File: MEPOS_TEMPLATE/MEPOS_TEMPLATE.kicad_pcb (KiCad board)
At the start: 4 copper layers, 101.6 x 101.6 mm, 10 parts, among them J201 Conn_02x32_Odd_Even, J202 Conn_02x20_Odd_Even

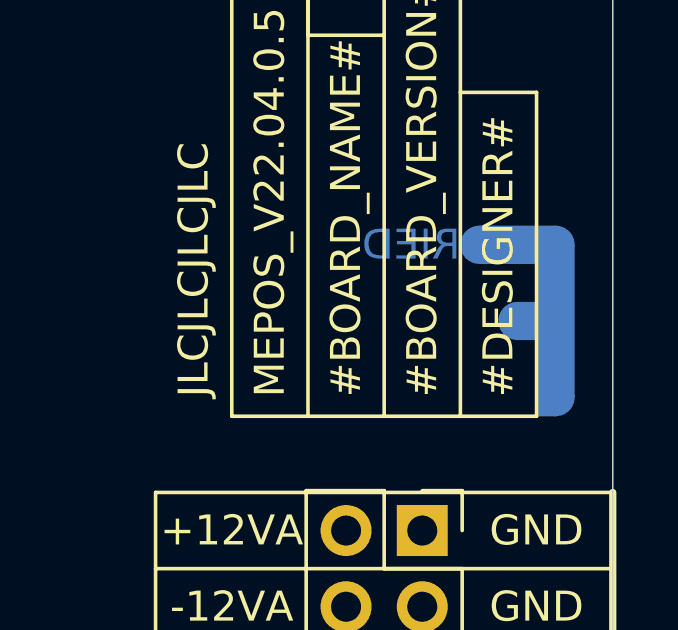
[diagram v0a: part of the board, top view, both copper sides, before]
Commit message: Updated Libraries
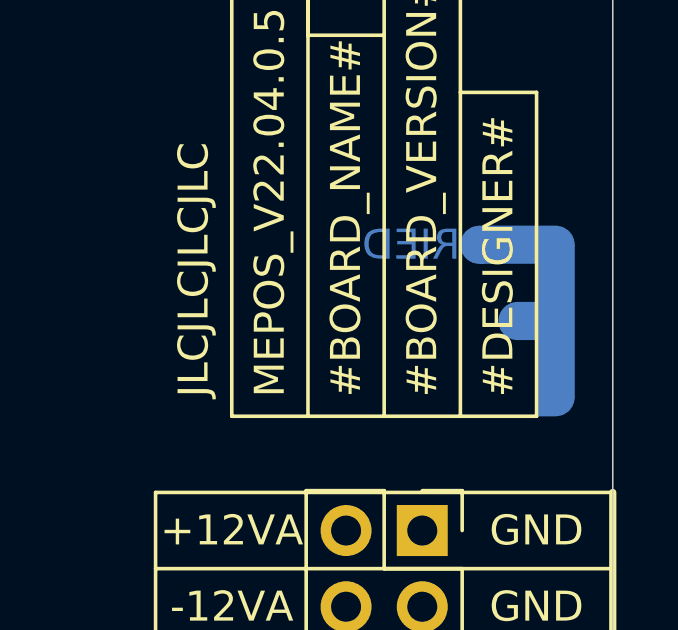
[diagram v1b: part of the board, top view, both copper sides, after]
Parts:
- removed the REF** at (188.1, 68.9)
- added REF**: Logo, MEPOS:Logo, F.Cu at (188.1, 68.9)
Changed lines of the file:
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@@
     )
   )
-  (footprint "MEP_TEMPLATE:Logo" (layer "F.Cu")
-    (at 188.09775 68.885)
+  (footprint "MEPOS:Logo" (layer "F.Cu")
+    (at 188.1 68.885)
     (attr smd)
     (fp_text reference "REF**" (at 0 -4.445 unlocked) (layer "F.Fab")
@@
     )
     (fp_circle (center 3.175 -2.54) (end 3.81 -2.54) (layer "B.Cu") (width 0.001) (fill solid))
+    (fp_circle (center 4.445 0) (end 5.08 0) (layer "B.Cu") (width 0.001) (fill solid))
     (fp_circle (center 5.715 -2.54) (end 6.35 -2.54) (layer "B.Cu") (width 0.001) (fill solid))
-    (fp_circle (center 4.445 0) (end 5.08 0) (layer "B.Cu") (width 0.001) (fill solid))
     (fp_circle (center 5.715 2.54) (end 6.35 2.54) (layer "B.Cu") (width 0.001) (fill solid))
     (fp_poly (pts
@@
     (fp_circle (center 4.445 0) (end 5.08 0) (layer "B.Mask") (width 0.001) (fill solid))
     (fp_circle (center 5.715 -2.54) (end 6.35 -2.54) (layer "B.Mask") (width 0.001) (fill solid))
+    (fp_circle (center 3.175 -2.54) (end 3.81 -2.54) (layer "B.Mask") (width 0.001) (fill solid))
     (fp_circle (center 5.715 2.54) (end 6.35 2.54) (layer "B.Mask") (width 0.001) (fill solid))
-    (fp_circle (center 3.175 -2.54) (end 3.81 -2.54) (layer "B.Mask") (width 0.001) (fill solid))
     (fp_poly (pts
         (xy 6.35 -2.54)
